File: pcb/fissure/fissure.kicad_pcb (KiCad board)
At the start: 2 copper layers, 99.5 x 95 mm, 45 parts, among them J1 AudioJack4, J2 AudioJack4, K1 KEYSW, K10 KEYSW, K11 KEYSW, K12 KEYSW, K13 KEYSW, K14 KEYSW, K15 KEYSW, K16 KEYSW, K17 KEYSW, K18 KEYSW, K2 KEYSW, K3 KEYSW, K4 KEYSW, K5 KEYSW, K6 KEYSW, K7 KEYSW, K8 KEYSW, K9 KEYSW, SW1 SW_PUSH, U1 NRF24L01_Breakout, U3 ProMicro

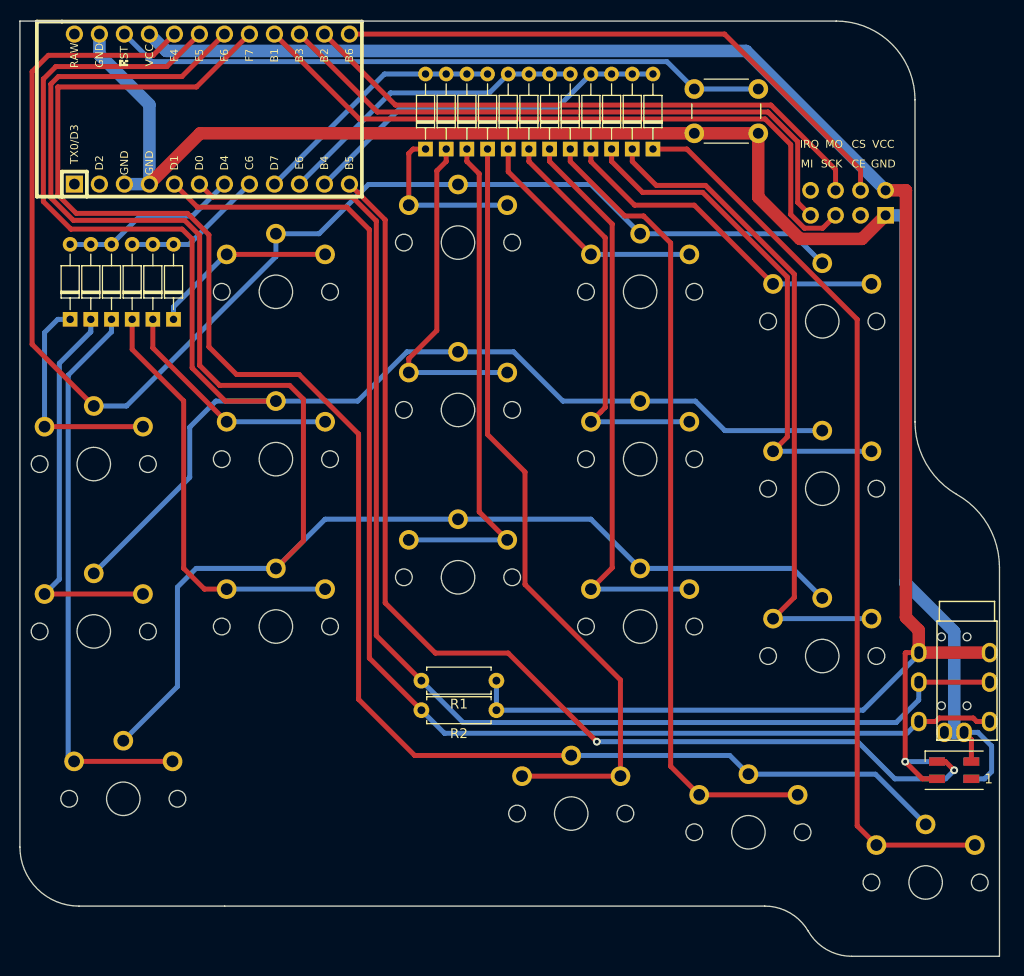
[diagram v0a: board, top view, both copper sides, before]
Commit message: v2.1 final
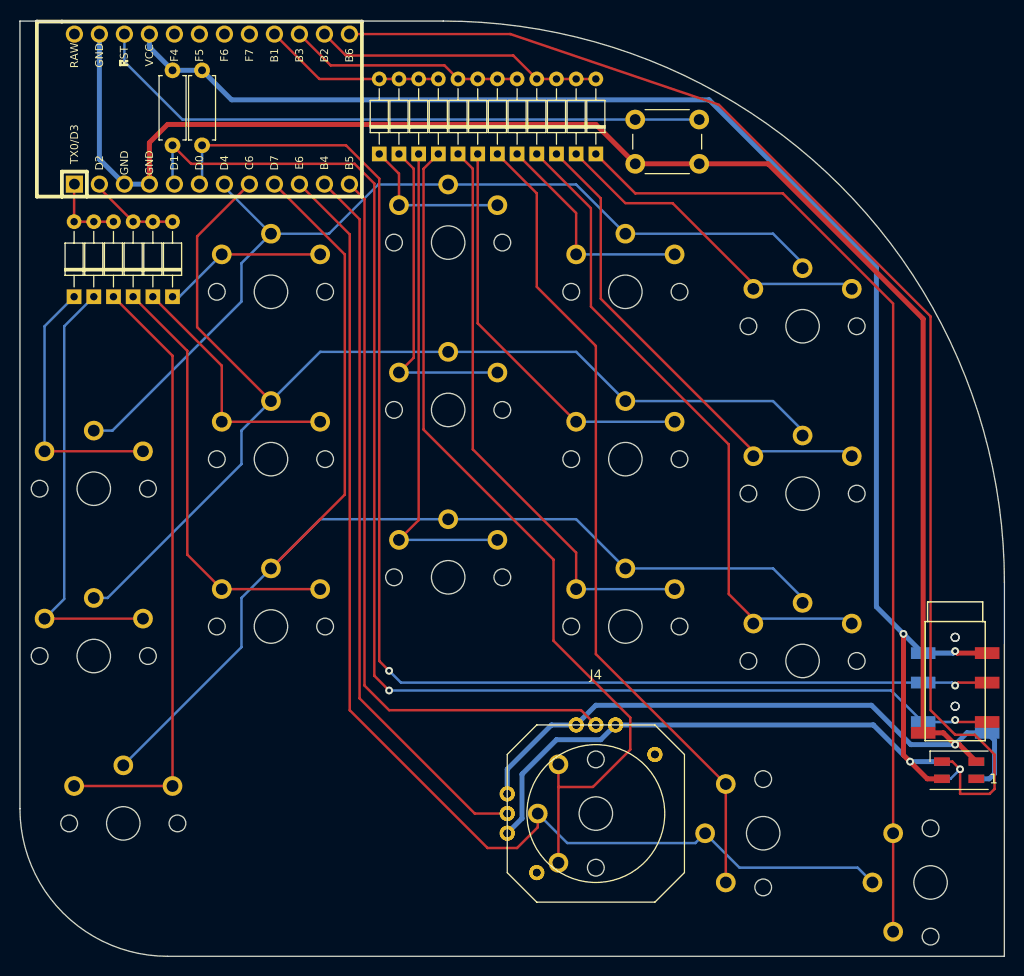
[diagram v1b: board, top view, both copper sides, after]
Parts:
- removed U1: NRF24L01_Breakout, Connector_PinHeader_2.54mm:PinHeader_2x04_P2.54mm_Vertical
- added J3: joystick, footprints:joystick, B.Cu at (102.5, 120.2)
- added J4: joystick, footprints:joystick, F.Cu at (102.5, 120.2)
- J1, J2: footprint Keebio-Parts:TRRS-PJ-320A -> Keebio-Parts:TRRS-PJ-320D
- moved R2 72.9 mm to (59.5, 44.7), turned to 270 degrees
- moved R1 68.8 mm to (62.5, 44.7), turned to 270 degrees
- moved D15 9.71 mm to (96.5, 53.2)
- moved D14 9.31 mm to (88.5, 53.2)
- moved D17 7.42 mm to (92.5, 53.2)
- moved SW1 6.75 mm to (113.0, 54.2)
- moved D18 5.82 mm to (102.5, 53.2)
- moved D10 5.62 mm to (98.5, 53.2)
- moved D9 5.22 mm to (90.5, 53.2)
- moved D16 5.02 mm to (86.5, 53.2)
- moved D13 4.93 mm to (84.5, 53.2)
- moved D8 4.83 mm to (82.5, 53.2)
- moved D3 4.73 mm to (80.5, 53.2)
- moved K1 2.50 mm to (51.5, 87.2)
- moved K11 2.50 mm to (54.5, 121.2)
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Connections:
- U3 pad 1: TX -> COL1
- U3 pad 10: COL4 -> ROW4
- U3 pad 11: COL5 -> X
- U3 pad 12: RGB -> Y
- U3 pad 13: CS -> RGB
- U3 pad 14: MOSI -> COL5
- U3 pad 15: MISO -> COL4
- U3 pad 16: SCLK -> COL3
- U3 pad 17: ROW4 -> Net-(U3-Pad17)
- U3 pad 18: ROW3 -> Net-(U3-Pad18)
- U3 pad 19: ROW2 -> Net-(U3-Pad19)
- U3 pad 2: RX -> COL2
- U3 pad 20: ROW1 -> Net-(U3-Pad20)
- U3 pad 7: COL1 -> ROW1
- U3 pad 8: COL2 -> ROW2
- U3 pad 9: COL3 -> ROW3
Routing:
- net Y: track 0.00 -> 76.7 mm
- net X: track 0.00 -> 73.6 mm
- net SCLK: track 69.9 -> 0.00 mm
- net MISO: track 63.2 -> 0.00 mm
- net MOSI: track 59.7 -> 0.00 mm
- net CS: track 59.7 -> 0.00 mm
- net ROW3: track 181.1 -> 130.7 mm
- net ROW4: track 169.8 -> 120.5 mm
- net ROW1: track 140.6 -> 95.0 mm
- net GND: track 176.4 -> 221.9 mm, vias 0 -> 1
- net ROW2: track 159.5 -> 115.0 mm
- net RGB: track 111.7 -> 131.6 mm, vias 2 -> 1
- net COL1: track 18.2 -> 7.83 mm
- net Net-(D16-Pad1): track 79.3 -> 88.7 mm
- net COL5: track 38.0 -> 29.5 mm
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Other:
- board size 99.5 x 95 mm -> 100 x 95 mm
- board text removed: "CE"
- board text removed: "CS"
- board text removed: "GND"
- board text removed: "IRQ"
- board text removed: "MI"
- board text removed: "MO"
- board text removed: "SCK"
- board text removed: "VCC"
